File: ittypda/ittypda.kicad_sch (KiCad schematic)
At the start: 151 parts, among them CN1 S2B-PH-SM4-TB, J1 USB_C_Receptacle_USB2.0_14P, J13 Conn_01x05_Pin, J14 Conn_01x05_Pin, J2 Conn_01x04_Pin, SW1 Switch, SW10 Switch, SW11 Switch, SW12 Switch, SW13 Switch, SW14 Switch, SW15 Switch, SW16 Switch, SW17 Switch, SW18 Switch, SW19 Switch, SW2 Switch, SW20 Switch, SW21 Switch, SW22 Switch, SW23 Switch, SW24 Switch, SW25 SLIDE SWITCH, SW26 Switch, SW27 Switch, SW28 Switch, SW29 Switch, SW3 Switch, SW30 Switch, SW31 Switch, SW32 Switch, SW33 Switch, SW34 Switch, SW36 Switch, SW37 Switch, SW38 Switch, SW39 Switch, SW4 Switch, SW41 Switch, SW42 Switch, SW43 Switch, SW44 Switch, SW45 Switch, SW46 Switch, SW47 Switch, SW48 Switch, SW49 Switch, SW5 Switch, SW50 Switch, SW51 Switch, SW52 Switch, SW53 Switch, SW54 Switch, SW55 Switch, SW56 Switch, SW57 Switch, SW58 Switch, SW59 Switch, SW6 Switch, SW60 Switch, SW61 Switch, SW7 Switch, SW8 Switch, SW9 Switch, U1 STM32F401RETx, U2 BQ24040DSQR, U3 TLV75801PDRV, Y1 16Mhz

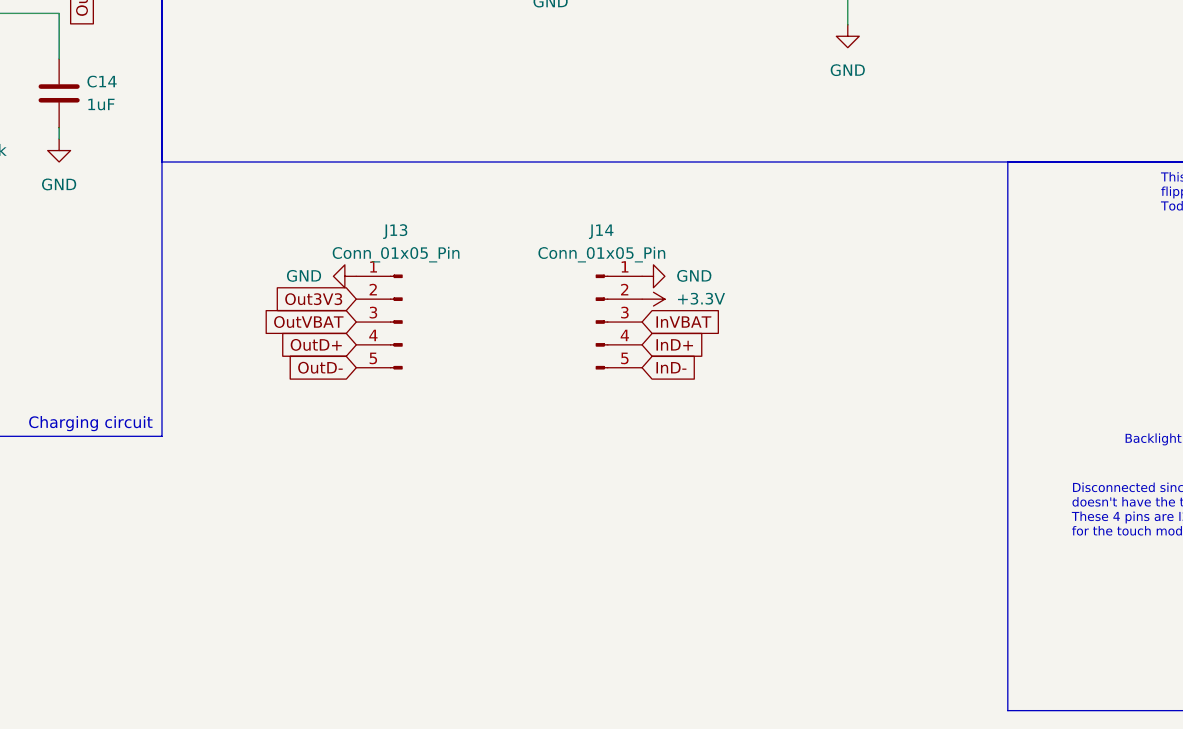
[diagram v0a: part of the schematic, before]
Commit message: organize schem
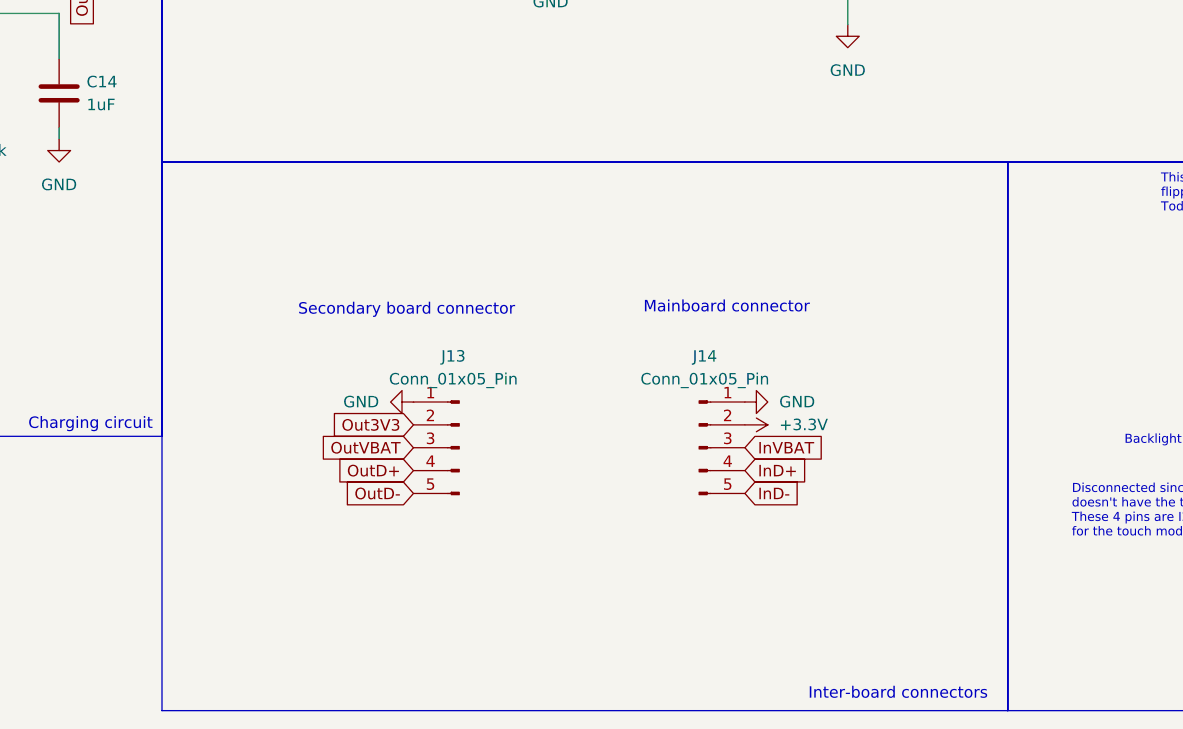
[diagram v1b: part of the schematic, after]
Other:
- note added: "Inter-board connectors"
- note added: "Mainboard connector"
- note added: "Secondary board connector"
- moved on the sheet: J13, J14
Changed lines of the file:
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@@
 	)
 	(rectangle
+		(start 236.22 190.5)
+		(end 330.2 251.46)
+		(stroke
+			(width 0)
+			(type default)
+		)
+		(fill
+			(type none)
+		)
+	)
+	(rectangle
 		(start 236.22 58.42)
 		(end 391.16 190.5)
@@
 		)
 	)
+	(text "Secondary board connector"
+		(exclude_from_sim no)
+		(at 263.398 207.01 0)
+		(effects
+			(font
+				(size 1.27 1.27)
+			)
+		)
+	)
 	(text "Microcontroller"
 		(exclude_from_sim no)
@@
 		)
 	)
+	(text "Inter-board connectors"
+		(exclude_from_sim no)
+		(at 318.008 249.682 0)
+		(effects
+			(font
+				(size 1.27 1.27)
+			)
+		)
+	)
 	(text "Debug pins"
 		(exclude_from_sim no)
@@
 		)
 	)
+	(text "Mainboard connector"
+		(exclude_from_sim no)
+		(at 298.958 206.756 0)
+		(effects
+			(font
+				(size 1.27 1.27)
+			)
+		)
+	)
 	(text "Decouplers"
 		(exclude_from_sim no)
@@
 	(global_label "Out3V3"
 		(shape input)
-		(at 257.81 205.74 180)
+		(at 264.16 219.71 180)
 		(fields_autoplaced yes)
 		(effects
@@
 		)
 		(property "Intersheetrefs" "${INTERSHEET_REFS}"
-			(at 248.112 205.74 0)
+			(at 254.462 219.71 0)
 			(hide yes)
 			(show_name no)
@@
 	(global_label "InD+"
 		(shape input)
-		(at 289.56 210.82 0)
+		(at 300.99 224.79 0)
 		(fields_autoplaced yes)
 		(effects
@@
 		)
 		(property "Intersheetrefs" "${INTERSHEET_REFS}"
-			(at 297.1414 210.82 0)
+			(at 308.5714 224.79 0)
 			(hide yes)
 			(show_name no)
@@
 	(global_label "OutVBAT"
 		(shape input)
-		(at 257.81 208.28 180)
+		(at 264.16 222.25 180)
 		(fields_autoplaced yes)
 		(effects
@@
 		)
 		(property "Intersheetrefs" "${INTERSHEET_REFS}"
-			(at 247.2048 208.28 0)
+			(at 253.5548 222.25 0)
 			(hide yes)
 			(show_name no)
@@
 	(global_label "OutD-"
 		(shape input)
-		(at 257.81 213.36 180)
+		(at 264.16 227.33 180)
 		(fields_autoplaced yes)
 		(effects
@@
 		)
 		(property "Intersheetrefs" "${INTERSHEET_REFS}"
-			(at 248.7772 213.36 0)
+			(at 255.1272 227.33 0)
 			(hide yes)
 			(show_name no)
@@
 	(global_label "InD-"
 		(shape input)
-		(at 289.56 213.36 0)
+		(at 300.99 227.33 0)
 		(fields_autoplaced yes)
 		(effects
@@
 		)
 		(property "Intersheetrefs" "${INTERSHEET_REFS}"
-			(at 297.1414 213.36 0)
+			(at 308.5714 227.33 0)
 			(hide yes)
 			(show_name no)
@@
 	(global_label "InVBAT"
 		(shape input)
-		(at 289.56 208.28 0)
+		(at 300.99 222.25 0)
 		(fields_autoplaced yes)
 		(effects
@@
 		)
 		(property "Intersheetrefs" "${INTERSHEET_REFS}"
-			(at 298.7138 208.28 0)
+			(at 310.1438 222.25 0)
 			(hide yes)
 			(show_name no)
@@
 	(global_label "OutD+"
 		(shape input)
-		(at 257.81 210.82 180)
+		(at 264.16 224.79 180)
 		(fields_autoplaced yes)
 		(effects
@@
 		)
 		(property "Intersheetrefs" "${INTERSHEET_REFS}"
-			(at 248.7772 210.82 0)
+			(at 255.1272 224.79 0)
 			(hide yes)
 			(show_name no)
@@
 	(symbol
 		(lib_id "Connector:Conn_01x05_Pin")
-		(at 284.48 208.28 0)
+		(at 295.91 222.25 0)
 		(unit 1)
 		(body_style 1)
@@
 		(fields_autoplaced yes)
 		(property "Reference" "J14"
-			(at 285.115 198.12 0)
+			(at 296.545 212.09 0)
 			(show_name no)
 			(do_not_autoplace no)
@@
 		)
 		(property "Value" "Conn_01x05_Pin"
-			(at 285.115 200.66 0)
+			(at 296.545 214.63 0)
 			(show_name no)
 			(do_not_autoplace no)
@@
 		)
 		(property "Footprint" "Connector_PinHeader_2.54mm:PinHeader_1x05_P2.54mm_Vertical"
-			(at 284.48 208.28 0)
+			(at 295.91 222.25 0)
 			(hide yes)
 			(show_name no)
@@
 		)
 		(property "Datasheet" ""
-			(at 284.48 208.28 0)
+			(at 295.91 222.25 0)
 			(hide yes)
 			(show_name no)
@@
 		)
 		(property "Description" "Generic connector, single row, 01x05, script generated"
-			(at 284.48 208.28 0)
+			(at 295.91 222.25 0)
 			(hide yes)
 			(show_name no)
@@
 	(symbol
 		(lib_id "power:GND")
-		(at 257.81 203.2 270)
+		(at 264.16 217.17 270)
 		(unit 1)
 		(body_style 1)
@@
 		(fields_autoplaced yes)
 		(property "Reference" "#PWR021"
-			(at 251.46 203.2 0)
+			(at 257.81 217.17 0)
 			(hide yes)
 			(show_name no)
@@
 		)
 		(property "Value" "GND"
-			(at 254 203.1999 90)
+			(at 260.35 217.1699 90)
 			(show_name no)
 			(do_not_autoplace no)
@@
 		)
 		(property "Footprint" ""
-			(at 257.81 203.2 0)
+			(at 264.16 217.17 0)
 			(hide yes)
 			(show_name no)
@@
 		)
 		(property "Datasheet" ""
-			(at 257.81 203.2 0)
+			(at 264.16 217.17 0)
 			(hide yes)
 			(show_name no)
@@
 		)
 		(property "Description" "Power symbol creates a global label with name \"GND\" , ground"
-			(at 257.81 203.2 0)
+			(at 264.16 217.17 0)
 			(hide yes)
 			(show_name no)
@@
 	(symbol
 		(lib_id "power:+3.3V")
-		(at 289.56 205.74 270)
+		(at 300.99 219.71 270)
 		(unit 1)
 		(body_style 1)
@@
 		(fields_autoplaced yes)
 		(property "Reference" "#PWR029"
-			(at 285.75 205.74 0)
+			(at 297.18 219.71 0)
 			(hide yes)
 			(show_name no)
@@
 		)
 		(property "Value" "+3.3V"
-			(at 293.37 205.7399 90)
+			(at 304.8 219.7099 90)
 			(show_name no)
 			(do_not_autoplace no)
@@
 		)
 		(property "Footprint" ""
-			(at 289.56 205.74 0)
+			(at 300.99 219.71 0)
 			(hide yes)
 			(show_name no)
@@
 		)
 		(property "Datasheet" ""
-			(at 289.56 205.74 0)
+			(at 300.99 219.71 0)
 			(hide yes)
 			(show_name no)
@@
 		)
 		(property "Description" "Power symbol creates a global label with name \"+3.3V\""
-			(at 289.56 205.74 0)
+			(at 300.99 219.71 0)
 			(hide yes)
 			(show_name no)
@@
 	(symbol
 		(lib_id "power:GND")
-		(at 289.56 203.2 90)
+		(at 300.99 217.17 90)
 		(unit 1)
 		(body_style 1)
@@
 		(fields_autoplaced yes)
 		(property "Reference" "#PWR028"
-			(at 295.91 203.2 0)
+			(at 307.34 217.17 0)
 			(hide yes)
 			(show_name no)
@@
 		)
 		(property "Value" "GND"
-			(at 293.37 203.1999 90)
+			(at 304.8 217.1699 90)
 			(show_name no)
 			(do_not_autoplace no)
@@
 		)
 		(property "Footprint" ""
-			(at 289.56 203.2 0)
+			(at 300.99 217.17 0)
 			(hide yes)
 			(show_name no)
@@
 		)
 		(property "Datasheet" ""
-			(at 289.56 203.2 0)
+			(at 300.99 217.17 0)
 			(hide yes)
 			(show_name no)
@@
 		)
 		(property "Description" "Power symbol creates a global label with name \"GND\" , ground"
-			(at 289.56 203.2 0)
+			(at 300.99 217.17 0)
 			(hide yes)
 			(show_name no)
@@
 	(symbol
 		(lib_id "Connector:Conn_01x05_Pin")
-		(at 262.89 208.28 0)
+		(at 269.24 222.25 0)
 		(mirror y)
 		(unit 1)
@@
 		(fields_autoplaced yes)
 		(property "Reference" "J13"
-			(at 262.255 198.12 0)
+			(at 268.605 212.09 0)
 			(show_name no)
 			(do_not_autoplace no)
@@
 		)
 		(property "Value" "Conn_01x05_Pin"
-			(at 262.255 200.66 0)
+			(at 268.605 214.63 0)
 			(show_name no)
 			(do_not_autoplace no)
@@
 		)
 		(property "Footprint" "Connector_PinHeader_2.54mm:PinHeader_1x05_P2.54mm_Vertical"
-			(at 262.89 208.28 0)
+			(at 269.24 222.25 0)
 			(hide yes)
 			(show_name no)
@@
 		)
 		(property "Datasheet" ""
-			(at 262.89 208.28 0)
+			(at 269.24 222.25 0)
 			(hide yes)
 			(show_name no)
@@
 		)
 		(property "Description" "Generic connector, single row, 01x05, script generated"
-			(at 262.89 208.28 0)
+			(at 269.24 222.25 0)
 			(hide yes)
 			(show_name no)
